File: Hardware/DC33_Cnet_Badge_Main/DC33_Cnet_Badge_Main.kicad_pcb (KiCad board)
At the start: 2 copper layers, 101 x 58 mm, 8 parts, among them J1 DC33_Cnet_Badge_SAO_Socket

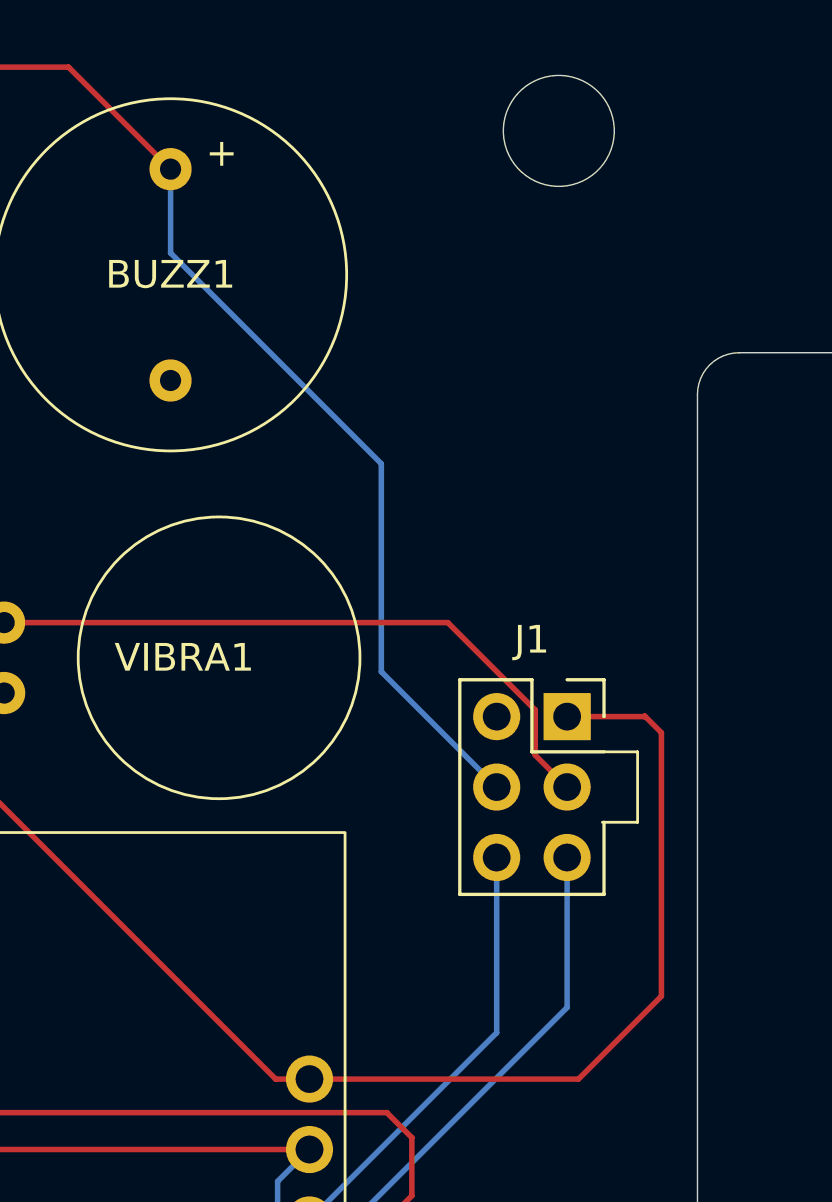
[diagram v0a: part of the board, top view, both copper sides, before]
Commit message: Case updates
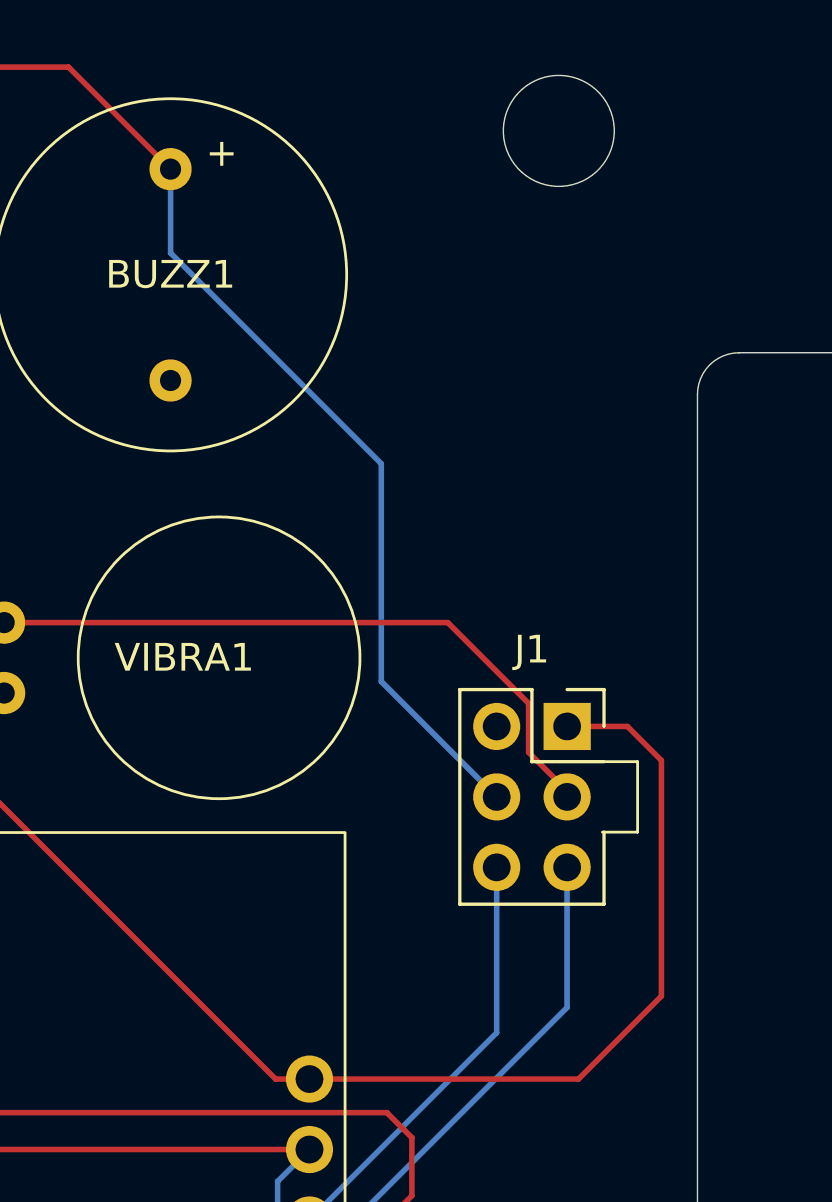
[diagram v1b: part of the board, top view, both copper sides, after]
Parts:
- moved J1 0.35 mm to (192.8, 78.0)
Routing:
- net 3V3: track 99.8 -> 99.1 mm
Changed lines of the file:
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@@
 	(footprint "DC33_Cnet_Badge_Main:DC33_Cnet_Badge_SAO_Socket"
 		(layer "F.Cu")
-		(at 192.8 77.62)
+		(at 192.8 77.975)
 		(descr "Through hole straight socket strip, 2x03, 2.54mm pitch, double cols (from Kicad 4.0.7), script generated")
 		(tags "Through hole socket strip THT 2x03 2.54mm double row")
@@
 	)
 	(segment
-		(start 186.1 68.5)
-		(end 186.1 76)
+		(start 178.5 60.9)
+		(end 178.5 57.88)
 		(width 0.2)
 		(layer "B.Cu")
@@
 	)
 	(segment
-		(start 178.5 60.9)
-		(end 186.1 68.5)
+		(start 190.26 80.515)
+		(end 186.1 76.355)
 		(width 0.2)
 		(layer "B.Cu")
@@
 	)
 	(segment
-		(start 178.5 57.88)
+		(start 186.1 68.5)
 		(end 178.5 60.9)
 		(width 0.2)
@@
 	)
 	(segment
-		(start 186.1 76)
-		(end 190.26 80.16)
+		(start 186.1 76.355)
+		(end 186.1 68.5)
 		(width 0.2)
 		(layer "B.Cu")
@@
 	(segment
 		(start 196.2 87.7)
-		(end 196.2 78.2)
+		(end 196.2 79.2)
 		(width 0.2)
 		(layer "F.Cu")
@@
 	)
 	(segment
-		(start 196.2 78.2)
-		(end 195.6 77.6)
+		(start 183.51 90.69)
+		(end 193.21 90.69)
 		(width 0.2)
 		(layer "F.Cu")
@@
 	)
 	(segment
-		(start 195.6 77.6)
-		(end 195.58 77.62)
+		(start 151.2 65.6)
+		(end 151.2 68.2)
+		(width 0.2)
+		(layer "F.Cu")
+		(net 3)
+	)
+	(segment
+		(start 182.29 90.69)
+		(end 183.51 90.69)
+		(width 0.2)
+		(layer "F.Cu")
+		(net 3)
+	)
+	(segment
+		(start 151.2 68.2)
+		(end 160.5 77.5)
+		(width 0.2)
+		(layer "F.Cu")
+		(net 3)
+	)
+	(segment
+		(start 126.4 56.64)
+		(end 129.26 59.5)
+		(width 0.2)
+		(layer "F.Cu")
+		(net 3)
+	)
+	(segment
+		(start 169.1 77.5)
+		(end 182.29 90.69)
+		(width 0.2)
+		(layer "F.Cu")
+		(net 3)
+	)
+	(segment
+		(start 196.2 79.2)
+		(end 194.975 77.975)
+		(width 0.2)
+		(layer "F.Cu")
+		(net 3)
+	)
+	(segment
+		(start 160.5 77.5)
+		(end 169.1 77.5)
+		(width 0.2)
+		(layer "F.Cu")
+		(net 3)
+	)
+	(segment
+		(start 194.975 77.975)
+		(end 192.8 77.975)
+		(width 0.2)
+		(layer "F.Cu")
+		(net 3)
+	)
+	(segment
+		(start 129.26 59.5)
+		(end 145.1 59.5)
 		(width 0.2)
 		(layer "F.Cu")
@@
 	)
 	(segment
-		(start 151.2 65.6)
-		(end 151.2 68.2)
-		(width 0.2)
-		(layer "F.Cu")
-		(net 3)
-	)
-	(segment
-		(start 182.29 90.69)
-		(end 183.51 90.69)
-		(width 0.2)
-		(layer "F.Cu")
-		(net 3)
-	)
-	(segment
-		(start 151.2 68.2)
-		(end 160.5 77.5)
-		(width 0.2)
-		(layer "F.Cu")
-		(net 3)
-	)
-	(segment
-		(start 126.4 56.64)
-		(end 129.26 59.5)
-		(width 0.2)
-		(layer "F.Cu")
-		(net 3)
-	)
-	(segment
-		(start 169.1 77.5)
-		(end 182.29 90.69)
-		(width 0.2)
-		(layer "F.Cu")
-		(net 3)
-	)
-	(segment
-		(start 183.51 90.69)
-		(end 193.21 90.69)
-		(width 0.2)
-		(layer "F.Cu")
-		(net 3)
-	)
-	(segment
-		(start 160.5 77.5)
-		(end 169.1 77.5)
-		(width 0.2)
-		(layer "F.Cu")
-		(net 3)
-	)
-	(segment
-		(start 129.26 59.5)
-		(end 145.1 59.5)
-		(width 0.2)
-		(layer "F.Cu")
-		(net 3)
-	)
-	(segment
-		(start 195.58 77.62)
-		(end 192.8 77.62)
-		(width 0.2)
-		(layer "F.Cu")
-		(net 3)
-	)
-	(segment
 		(start 145.1 59.5)
 		(end 151.2 65.6)
@@
 	)
 	(segment
-		(start 192.8 82.7)
-		(end 192.8 88.106346)
+		(start 192.8 88.106346)
+		(end 183.986346 96.92)
 		(width 0.2)
 		(layer "B.Cu")
@@
 	)
 	(segment
-		(start 192.8 88.106346)
-		(end 183.986346 96.92)
+		(start 183.986346 96.92)
+		(end 183.02 96.92)
 		(width 0.2)
 		(layer "B.Cu")
@@
 	)
 	(segment
-		(start 183.986346 96.92)
-		(end 183.02 96.92)
+		(start 192.8 88.106346)
+		(end 192.8 83.055)
 		(width 0.2)
 		(layer "B.Cu")
@@
 	)
 	(segment
-		(start 190.26 82.7)
-		(end 190.26 89.02)
+		(start 190.26 89.02)
+		(end 190.26 83.055)
 		(width 0.2)
 		(layer "B.Cu")
@@
 	)
 	(segment
-		(start 188.496346 74.23)
-		(end 191.65 77.383654)
+		(start 192.8 80.515)
+		(end 192.8 80.3)
 		(width 0.2)
 		(layer "F.Cu")
@@
 	)
 	(segment
-		(start 191.65 77.383654)
-		(end 191.65 79.01)
+		(start 192.8 80.3)
+		(end 191.41 78.91)
 		(width 0.2)
 		(layer "F.Cu")
@@
 	)
 	(segment
-		(start 191.65 79.01)
-		(end 192.8 80.16)
+		(start 191.41 77.143654)
+		(end 188.496346 74.23)
 		(width 0.2)
 		(layer "F.Cu")
@@
 		(width 0.2)
 		(layer "F.Cu")
+		(net 6)
+	)
+	(segment
+		(start 191.41 78.91)
+		(end 191.41 77.143654)
+		(width 0.2)
+		(layer "F.Cu")
